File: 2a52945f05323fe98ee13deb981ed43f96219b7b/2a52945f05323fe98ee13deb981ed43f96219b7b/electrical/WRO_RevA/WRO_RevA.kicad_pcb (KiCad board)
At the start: 2 copper layers, 75 x 57 mm, 0 parts

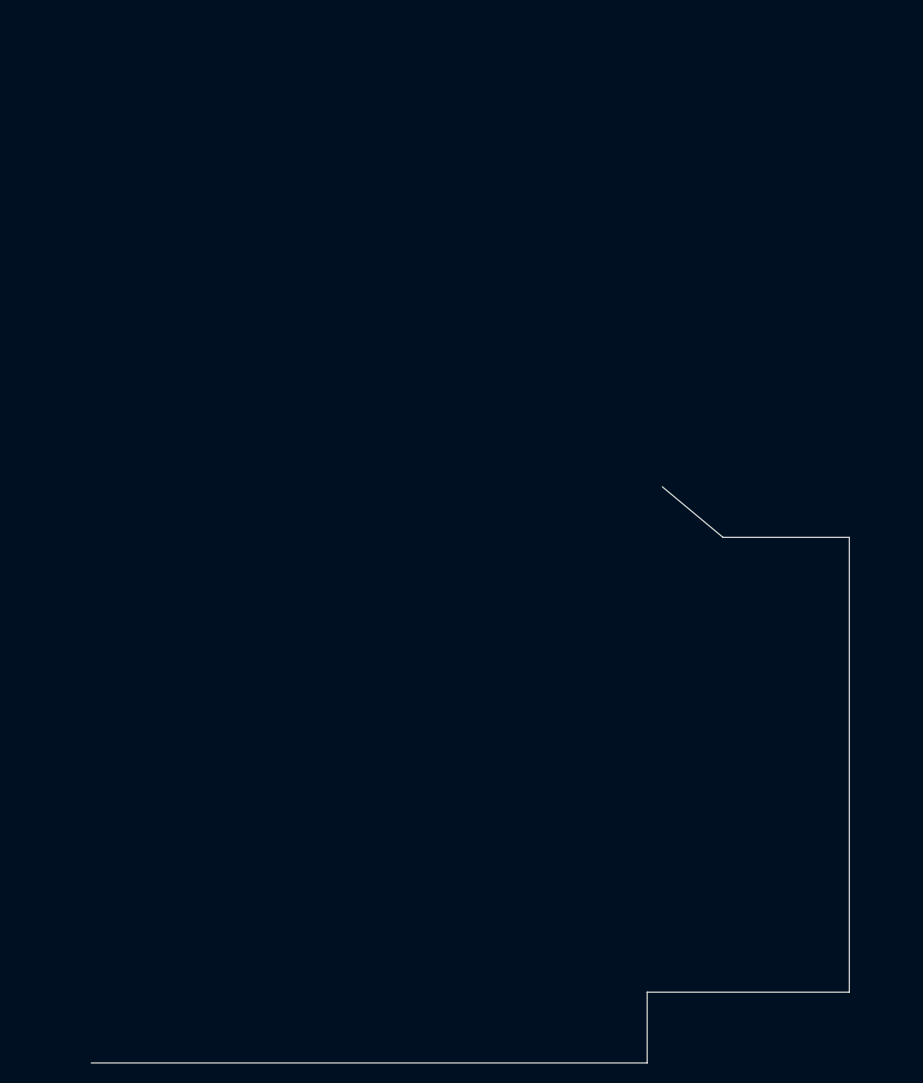
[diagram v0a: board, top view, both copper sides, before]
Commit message: final shape for PCB, only need to route
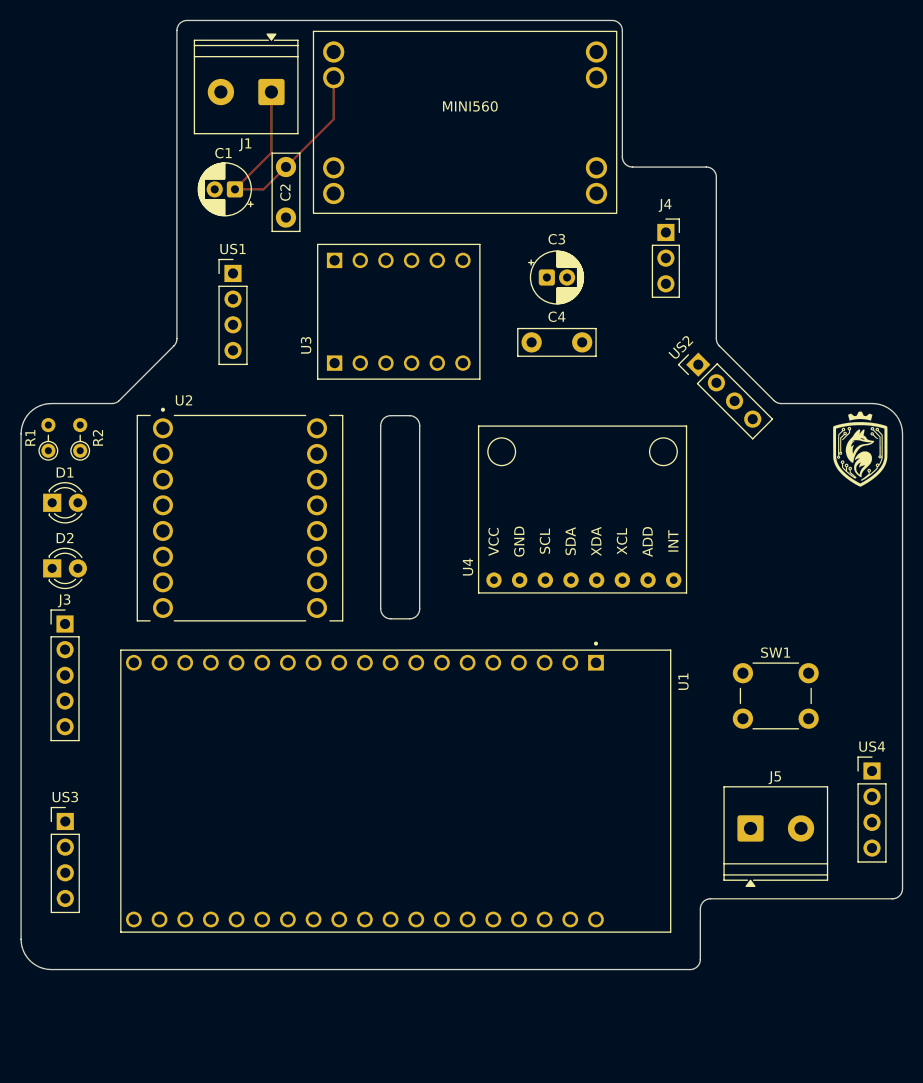
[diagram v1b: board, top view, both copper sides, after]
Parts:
- added C1: 470uF, Capacitor_THT:CP_Radial_D5.0mm_P2.00mm, F.Cu at (122.3, 45.6)
- added C2: 0.1uF, Capacitor_THT:C_Disc_D7.5mm_W2.5mm_P5.00mm, F.Cu at (127.4, 48.4)
- added C3: 470uF, Capacitor_THT:CP_Radial_D5.0mm_P2.00mm, F.Cu at (153.2, 54.4)
- added C4: 0.1uF, Capacitor_THT:C_Disc_D7.5mm_W2.5mm_P5.00mm, F.Cu at (151.7, 60.8)
- added D1: PWR, LED_THT:LED_D3.0mm, F.Cu at (104.3, 76.7)
- added D2: READY, LED_THT:LED_D3.0mm, F.Cu at (104.3, 83.2)
- added G***: LOGO, LogoFoxR_2:LogoFoxR_2, F.Cu at (184.2, 71.5)
- added J1: VCC, TerminalBlock_Phoenix:TerminalBlock_Phoenix_PT-1,5-2-5.0-H_1x02_P5.00mm_Horizontal, F.Cu at (126.0, 36.0)
- added J3: TO_PI, Connector_PinHeader_2.54mm:PinHeader_1x05_P2.54mm_Vertical, F.Cu at (105.5, 88.7)
- added J4: SERVO, Connector_PinSocket_2.54mm:PinSocket_1x03_P2.54mm_Vertical, F.Cu at (165.0, 49.9)
- added J5: MOTOR, TerminalBlock_Phoenix:TerminalBlock_Phoenix_PT-1,5-2-5.0-H_1x02_P5.00mm_Horizontal, F.Cu at (173.4, 108.9)
- added MINI560: V1, Libreria_mia:Mini560, F.Cu at (145.1, 39.0)
- added R1: 330, Resistor_THT:R_Axial_DIN0204_L3.6mm_D1.6mm_P2.54mm_Vertical, F.Cu at (103.9, 71.5)
- added R2: 330, Resistor_THT:R_Axial_DIN0204_L3.6mm_D1.6mm_P2.54mm_Vertical, F.Cu at (107.0, 71.5)
- added SW1: EXEC_PRGM, Button_Switch_THT:SW_PUSH_6mm, F.Cu at (172.6, 93.5)
- added U1: ESP32-DEVKITC-32D, ESP32-DEVKITC-32D:ESP32-DEVKITC-32D, F.Cu at (138.3, 105.2)
- added U2: ROB-14450, Snapeda:MODULE_ROB-14450, F.Cu at (122.8, 78.2)
- added U3: BOB-12009, Snapeda:CONV_BOB-12009, F.Cu at (138.6, 57.8)
- added U4: MPU6050, usini_sensors:module_mpu6050, F.Cu at (165.8, 84.3)
- added US1: ULTRASONIC, Connector_PinHeader_2.54mm:PinHeader_1x04_P2.54mm_Vertical, F.Cu at (122.2, 54.0)
- added US2: ULTRASONIC, Connector_PinHeader_2.54mm:PinHeader_1x04_P2.54mm_Vertical, F.Cu at (168.2, 63.0)
- added US3: ULTRASONIC, Connector_PinHeader_2.54mm:PinHeader_1x04_P2.54mm_Vertical, F.Cu at (105.6, 108.2)
- added US4: ULTRASONIC, Connector_PinHeader_2.54mm:PinHeader_1x04_P2.54mm_Vertical, F.Cu at (185.4, 103.2)
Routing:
- net +11.2V: track 0.00 -> 27.9 mm
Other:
- board size 75 x 57 mm -> 87.2 x 93.9 mm
